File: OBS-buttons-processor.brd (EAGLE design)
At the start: 144.8 x 81.2 mm, 23 parts

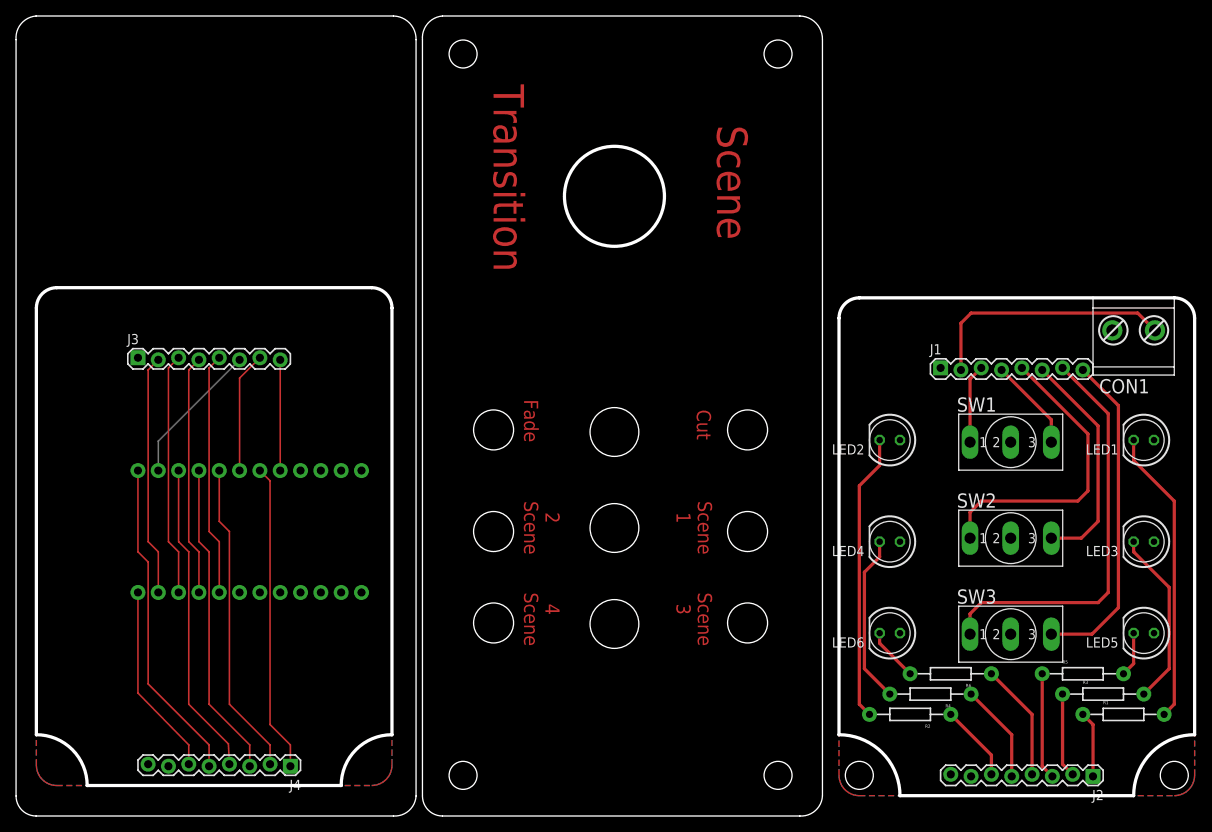
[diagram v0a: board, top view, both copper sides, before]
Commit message: initial prototype
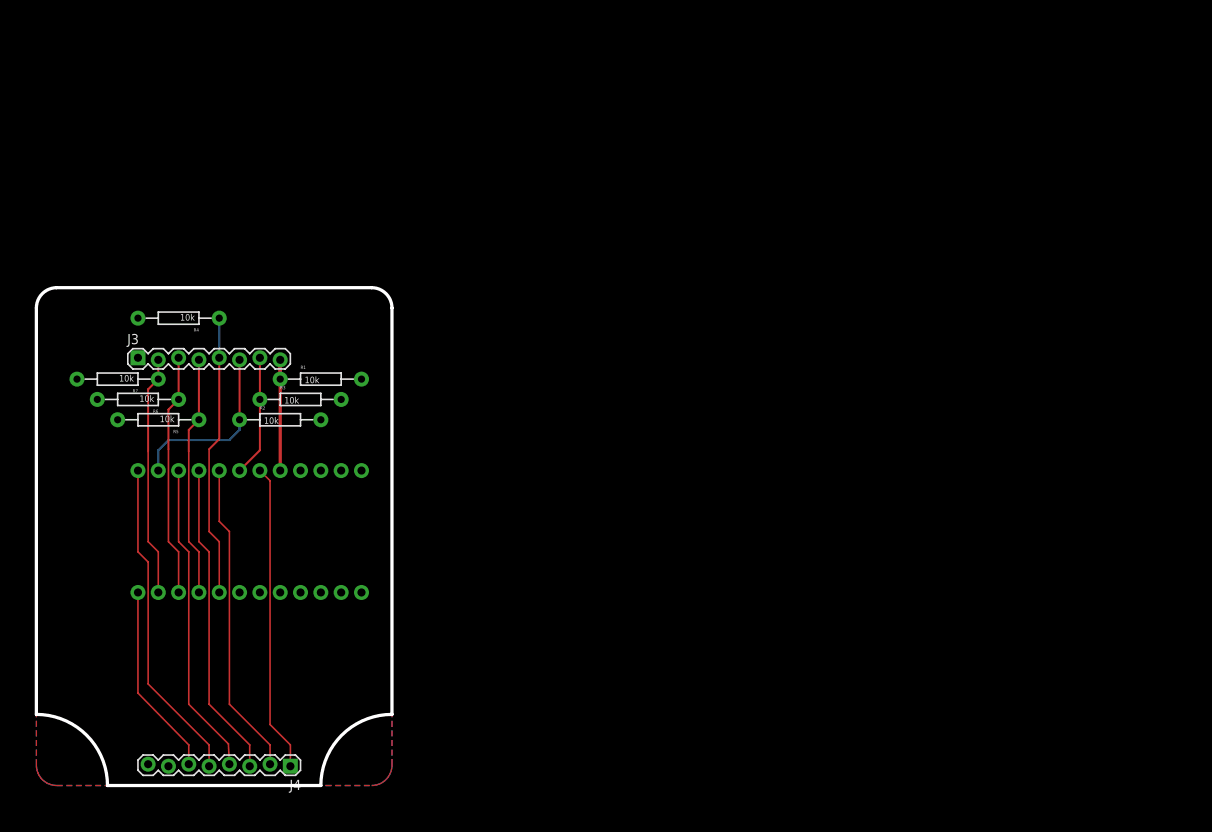
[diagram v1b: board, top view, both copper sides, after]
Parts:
- removed BOARD1, BOARD2: (no value), SPCoast:BOARD-SEEED10X5-NOHOLES
- removed CON1: (no value), SPCoast:MSTB2
- removed J1, J2: (no value), SPCoast:1X08_LOCK
- removed LED1, LED2, LED3, LED4, LED5, LED6: (no value), SPCoast:LED5MM
- removed SW1, SW2, SW3: (no value), SPCoast:SWITCH-SPDT-508
- added R7: 10k, SPCoast:AXIAL-0.4-RES
- R1, R2, R3, R4, R5, R6: value (none) -> 10k
- moved R5 119.9 mm to (17.8, 49.5), turned to 180 degrees
- moved R1 108.7 mm to (38.1, 54.6)
- moved R6 107.2 mm to (15.2, 52.1)
- moved R3 106.9 mm to (35.6, 52.1)
- moved R4 105.1 mm to (20.3, 62.2)
- moved R2 86.9 mm to (33.0, 49.5), turned to 0 degrees
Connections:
- removed net CUT: J1.3, SW1.1
- removed net CUT-LED: J2.1, R1.P$1
- removed net FADE: J1.4, SW1.3
- removed net FADE-LED: J2.6, R2.P$1
- removed net N$1: LED1.K, R1.P$2
- removed net N$2: LED2.K, R2.P$2
- removed net N$3: LED3.K, R3.P$2
- removed net N$4: LED4.K, R4.P$2
- removed net N$5: LED5.K, R5.P$2
- removed net N$6: LED6.K, R6.P$2
- removed net SCENE1: J1.5, SW2.1
- removed net SCENE1-LED: J2.2, R3.P$1
- removed net SCENE2: J1.6, SW2.3
- removed net SCENE2-LED: J2.5, R4.P$1
- removed net SCENE3: J1.7, SW3.1
- removed net SCENE3-LED: J2.3, R5.P$1
- removed net SCENE4: J1.8, SW3.3
- removed net SCENE4-LED: J2.4, R6.P$1
- removed net TRANSITION: CON1.2, J1.2
- net GND: no longer CON1.1, J2.7, J2.8, SW1.2, SW2.2, SW3.2
- net I1: now also R4.P$1
- net I2: now also R5.P$1
- net I3: now also R6.P$1
- net I4: now also R7.P$1
- net I5: now also R2.P$1
- net I6: now also R3.P$1
- net I7: now also R1.P$1
- net VCC: now also R1.P$2, R2.P$2, R3.P$2, R4.P$2, R5.P$2, R6.P$2, R7.P$2; no longer J1.1, LED1.A, LED2.A, LED3.A, LED4.A, LED5.A, LED6.A
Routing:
- net SCENE3: track 51.4 -> 0.00 mm
- net SCENE4: track 41.3 -> 0.00 mm
- net SCENE1: track 37.9 -> 0.00 mm
- net N$1: track 36.9 -> 0.00 mm
- net N$2: track 35.9 -> 0.00 mm
- net TRANSITION: track 31.5 -> 0.00 mm
- net SCENE2: track 28.5 -> 0.00 mm
- net N$3: track 22.2 -> 0.00 mm
- net N$4: track 21.2 -> 0.00 mm
- net SCENE4-LED: track 14.7 -> 0.00 mm
- net SCENE3-LED: track 13.4 -> 0.00 mm
- net SCENE2-LED: track 12.4 -> 0.00 mm
- net FADE: track 11.6 -> 0.00 mm
- net SCENE1-LED: track 10.6 -> 0.00 mm
- net CUT: track 9.86 -> 0.00 mm
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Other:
- board size 144.8 x 81.2 mm -> 44.5 x 62.2 mm
- board text removed: "2 Scene"
- board text removed: "4 Scene"
- board text removed: "Cut"
- board text removed: "Fade"
- board text removed: "Scene"
- board text removed: "Scene 1"
- board text removed: "Scene 3"
- board text removed: "Transition"
